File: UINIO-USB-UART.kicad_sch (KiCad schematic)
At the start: 4 parts

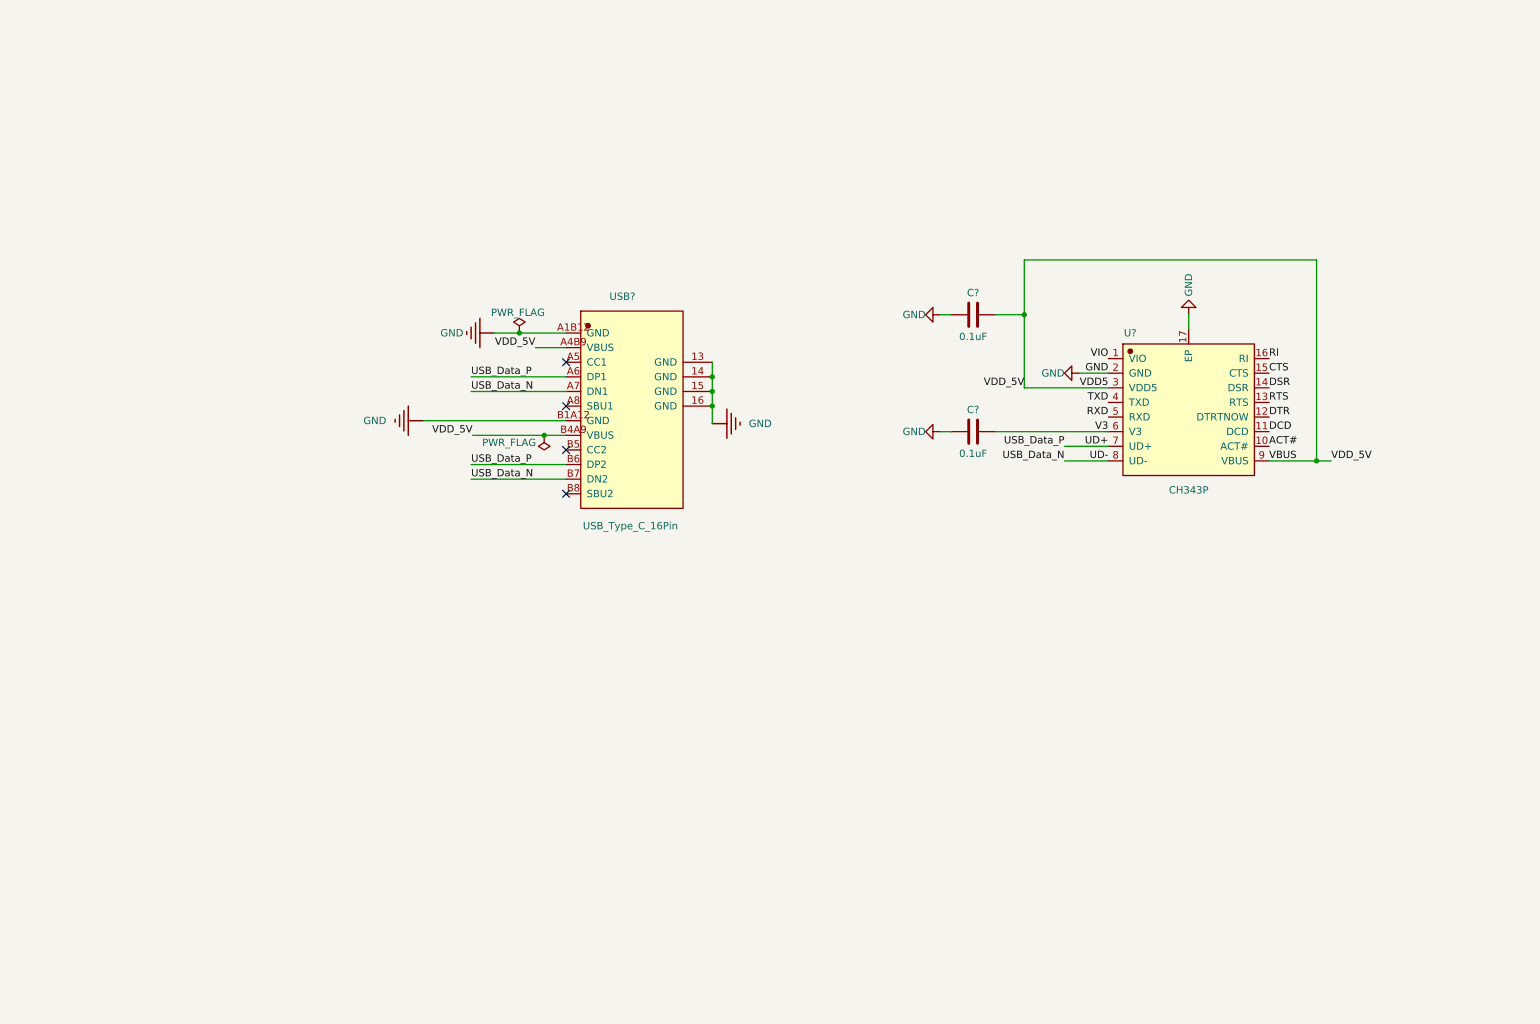
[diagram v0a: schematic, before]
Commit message: Finish the schematic diagram.
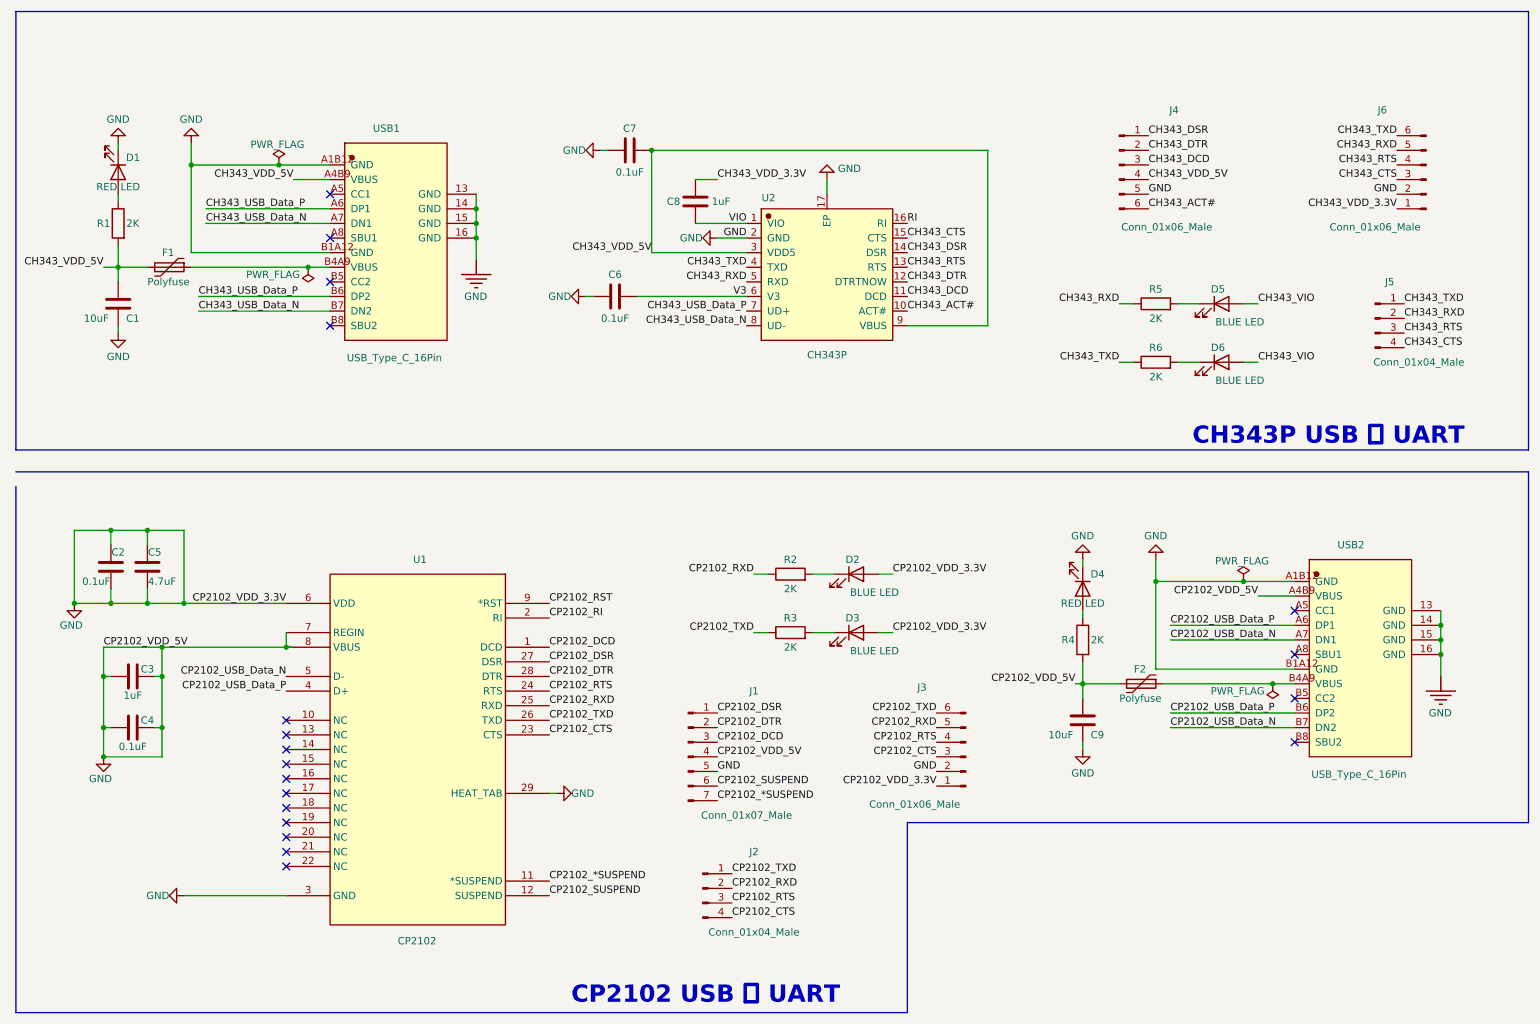
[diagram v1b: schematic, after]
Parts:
- added C1, C9: 10uF, symbol Device:C
- added C2, C4: 0.1uF, symbol Device:C
- added C3, C8: 1uF, symbol Device:C
- added C5: 4.7uF, symbol Device:C
- added D1, D4: RED LED, LED_SMD:LED_0603_1608Metric, symbol Device:LED
- added D2, D3, D5, D6: BLUE LED, symbol Device:LED
- added F1, F2: Polyfuse, Fuse:Fuse_1206_3216Metric, symbol Device:Polyfuse
- added J1: Conn_01x07_Male, symbol Connector:Conn_01x07_Male
- added J2, J5: Conn_01x04_Male, symbol Connector:Conn_01x04_Male
- added J3, J4, J6: Conn_01x06_Male, symbol Connector:Conn_01x06_Male
- added R1, R4: 2K, Resistor_SMD:R_0402_1005Metric, symbol Device:R
- added R2, R3, R5, R6: 2K, symbol Device:R
- added U1: CP2102, Uinio:QFN-28_L5.0-W5.0-P0.50-TL-EP3.3, symbol Uinio:CP2102
- added USB2: USB_Type_C_16Pin, Uinio:USB-C-SMD_TYPEC-304J-BCP16, symbol Uinio:USB_Type_C_16Pin
- gave numbers to parts that had none: 4
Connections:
- net GND: now also C1.2, C2.1, C2.2, C3.1, C3.2, C4.1, C4.2, C5.1, C5.2, C9.1, C9.2, D1.1 (K), D2.2 (A), D3.2 (A), D4.1 (K), F2.2, J1.4 (Pin_4), J1.5 (Pin_5), J3.1 (Pin_1), J3.2 (Pin_2), J4.5 (Pin_5), J6.2 (Pin_2), R4.2, U1.29 (HEAT_TAB), U1.3 (GND), U1.6 (VDD), U1.7 (REGIN), U1.8 (VBUS), USB2.13 (GND), USB2.14 (GND), USB2.15 (GND), USB2.16 (GND), USB2.A1B12 (GND), USB2.A4B9 (VBUS), USB2.B1A12 (GND)
- net VIO: now also C8.1
- net ACT# renamed CH343_ACT#
- net CH343_ACT#: now also J4.6 (Pin_6)
- net CTS renamed CH343_CTS
- net CH343_CTS: now also J5.4 (Pin_4), J6.3 (Pin_3)
- net DCD renamed CH343_DCD
- net CH343_DCD: now also J4.3 (Pin_3)
- net DSR renamed CH343_DSR
- net CH343_DSR: now also J4.1 (Pin_1)
- net DTR renamed CH343_DTR
- net CH343_DTR: now also J4.2 (Pin_2)
- net RTS renamed CH343_RTS
- net CH343_RTS: now also J5.3 (Pin_3), J6.4 (Pin_4)
- net RXD renamed CH343_RXD
- net CH343_RXD: now also J5.2 (Pin_2), J6.5 (Pin_5), R5.1
- net TXD renamed CH343_TXD
- net CH343_TXD: now also J5.1 (Pin_1), J6.6 (Pin_6), R6.1
- net UD+ renamed CH343_USB_Data_P
- net UD- renamed CH343_USB_Data_N
- net VBUS renamed CH343_VDD_5V
- net CH343_VDD_5V: now also C1.1, F1.2, J4.4 (Pin_4), R1.2; no longer USB1.B4A9 (VBUS)
- new net: D3.1 (K), R3.2
- new net: D2.1 (K), R2.2
- new net: D4.2 (A), R4.1
- new net: D1.2 (A), R1.1
- new net: D5.1 (K), R5.2
- new net: F2.1, USB2.B4A9 (VBUS)
- new net: D6.1 (K), R6.2
- new net: F1.1, USB1.B4A9 (VBUS)
- new net CH343_VDD_3.3V: C8.2, J6.1 (Pin_1)
- new net CH343_VIO: D5.2 (A), D6.2 (A)
- new net CP2102_*SUSPEND: J1.7 (Pin_7), U1.11 (*SUSPEND)
- new net CP2102_CTS: J2.4 (Pin_4), J3.3 (Pin_3), U1.23 (CTS)
- new net CP2102_DCD: J1.3 (Pin_3), U1.1 (DCD)
- new net CP2102_DSR: J1.1 (Pin_1), U1.27 (DSR)
- new net CP2102_DTR: J1.2 (Pin_2), U1.28 (DTR)
- new net CP2102_RI: U1.2 (RI)
- new net CP2102_RST: U1.9 (*RST)
- new net CP2102_RTS: J2.3 (Pin_3), J3.4 (Pin_4), U1.24 (RTS)
- new net CP2102_RXD: J2.2 (Pin_2), J3.5 (Pin_5), R2.1, U1.25 (RXD)
- new net CP2102_SUSPEND: J1.6 (Pin_6), U1.12 (SUSPEND)
- new net CP2102_TXD: J2.1 (Pin_1), J3.6 (Pin_6), R3.1, U1.26 (TXD)
- new net CP2102_USB_Data_N: U1.5 (D-), USB2.A7 (DN1), USB2.B7 (DN2)
- new net CP2102_USB_Data_P: U1.4 (D+), USB2.A6 (DP1), USB2.B6 (DP2)
- no-connect marks 4 -> 19
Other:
- note added: "CH343P USB 转 UART"
- note added: "CP2102 USB 转 UART"
- moved on the sheet: C6, C7, U2, USB1
